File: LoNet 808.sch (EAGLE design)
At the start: 39 parts, among them CN2 JST-2.0, IC1 LM2596S, J4 MICRO-SMD, J5 DC-005, U1 TXB0104PWR, U3 ATMEGA328P-AU-TQFP32

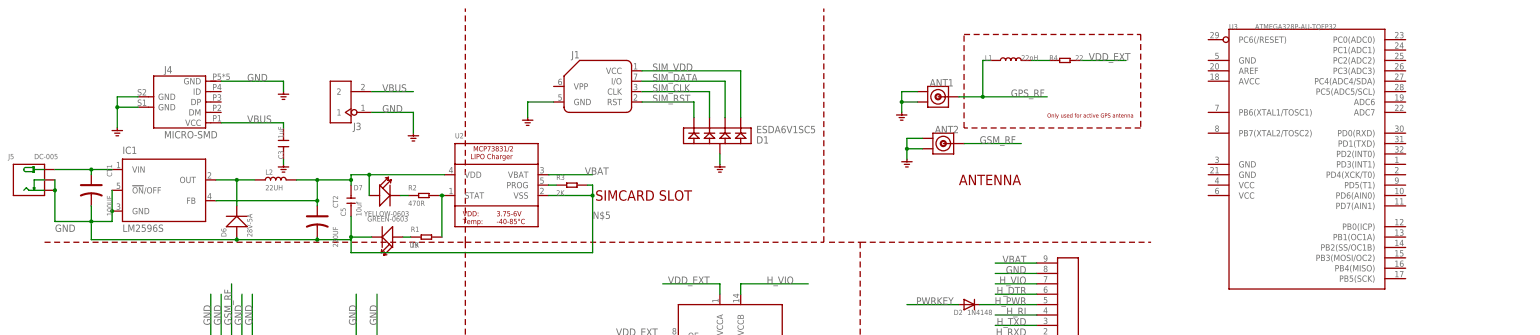
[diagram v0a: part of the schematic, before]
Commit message: more connection
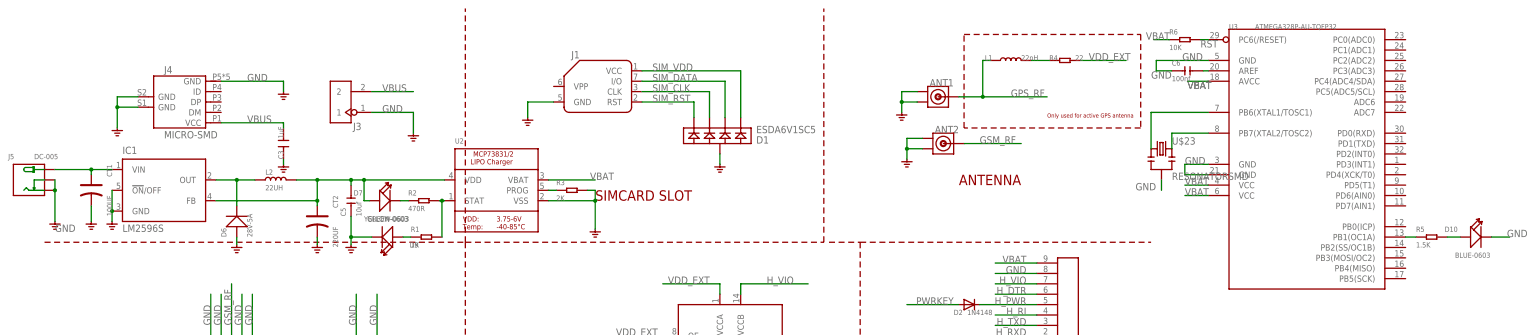
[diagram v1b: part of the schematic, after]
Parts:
- added C6: 100nf, Seeed-OPL-Capacitor:CERAMIC-100NF-50V-10%-X7R(0603)
- added D10: BLUE-0603, Seeed-OPL-Diode:SMD-LED-CLEAR-BLUE(0603)
- added R5: 1.5K, Seeed-OPL-Resistor:SMD-RES-1.5K-1%-1/10W(0603)
- added R6: 10K, Seeed-OPL-Resistor:SMD-RES-10K-1%-1/10W(0603)
- added U$23: RESONATORSMD, SparkFun:RESONATORSMD
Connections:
- removed net N$5 (its old number): C5.1, CT2.-, D6.+, D9.-, R3.2, U2.VSS
- new net N$11: C6.2, U3.AREF
- new net N$13: R5.1, U3.PB1(OC1A)
- new net N$14: D10.+, R5.2
- new net N$15: U$23.1, U3.PB6(XTAL1/TOSC1)
- new net N$16: U$23.3, U3.PB7(XTAL2/TOSC2)
- new net RST: R6.2, U3.PC6(/RESET)
- net GND: now also C5.1, C6.1, CT2.-, D10.-, D6.+, D9.-, R3.2, U$23.2, U2.VSS, U3.GND, U3.GND@1, U3.GND@2
- net VBAT: now also R6.1, U3.AVCC, U3.VCC@1, U3.VCC@2
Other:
- moved on the sheet: D7, R2, R3, U2
